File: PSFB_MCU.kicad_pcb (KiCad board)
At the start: 4 copper layers, 122.5 x 123.5 mm, 296 parts, among them Y1 16M

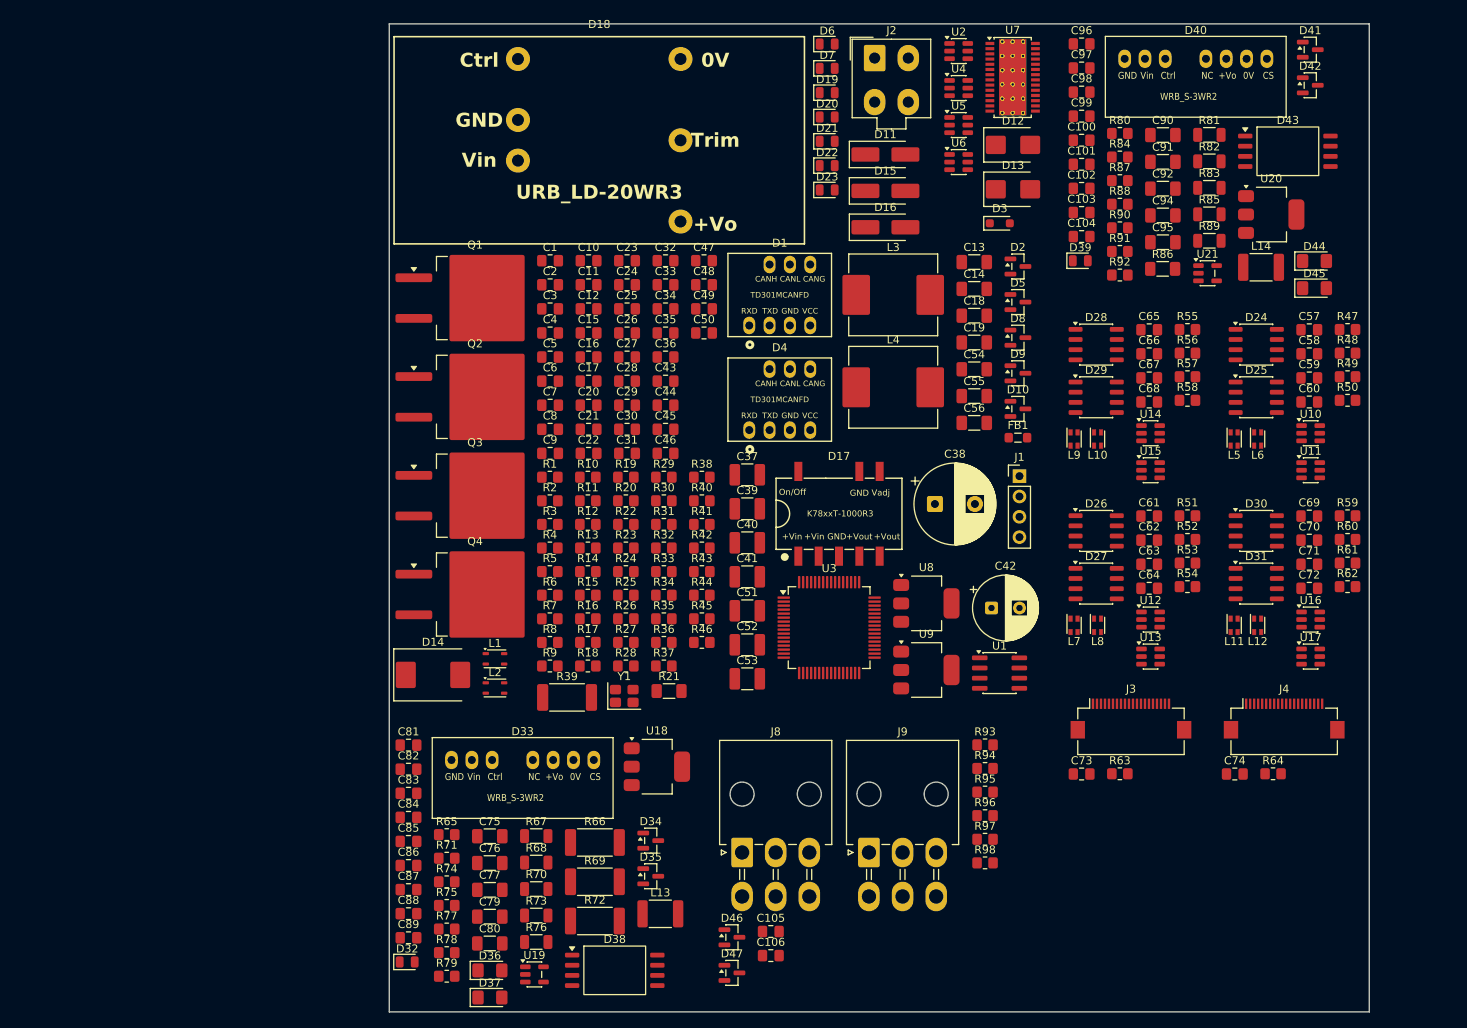
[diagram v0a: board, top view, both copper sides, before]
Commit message: VER1.0: раскидал компоненты на плате
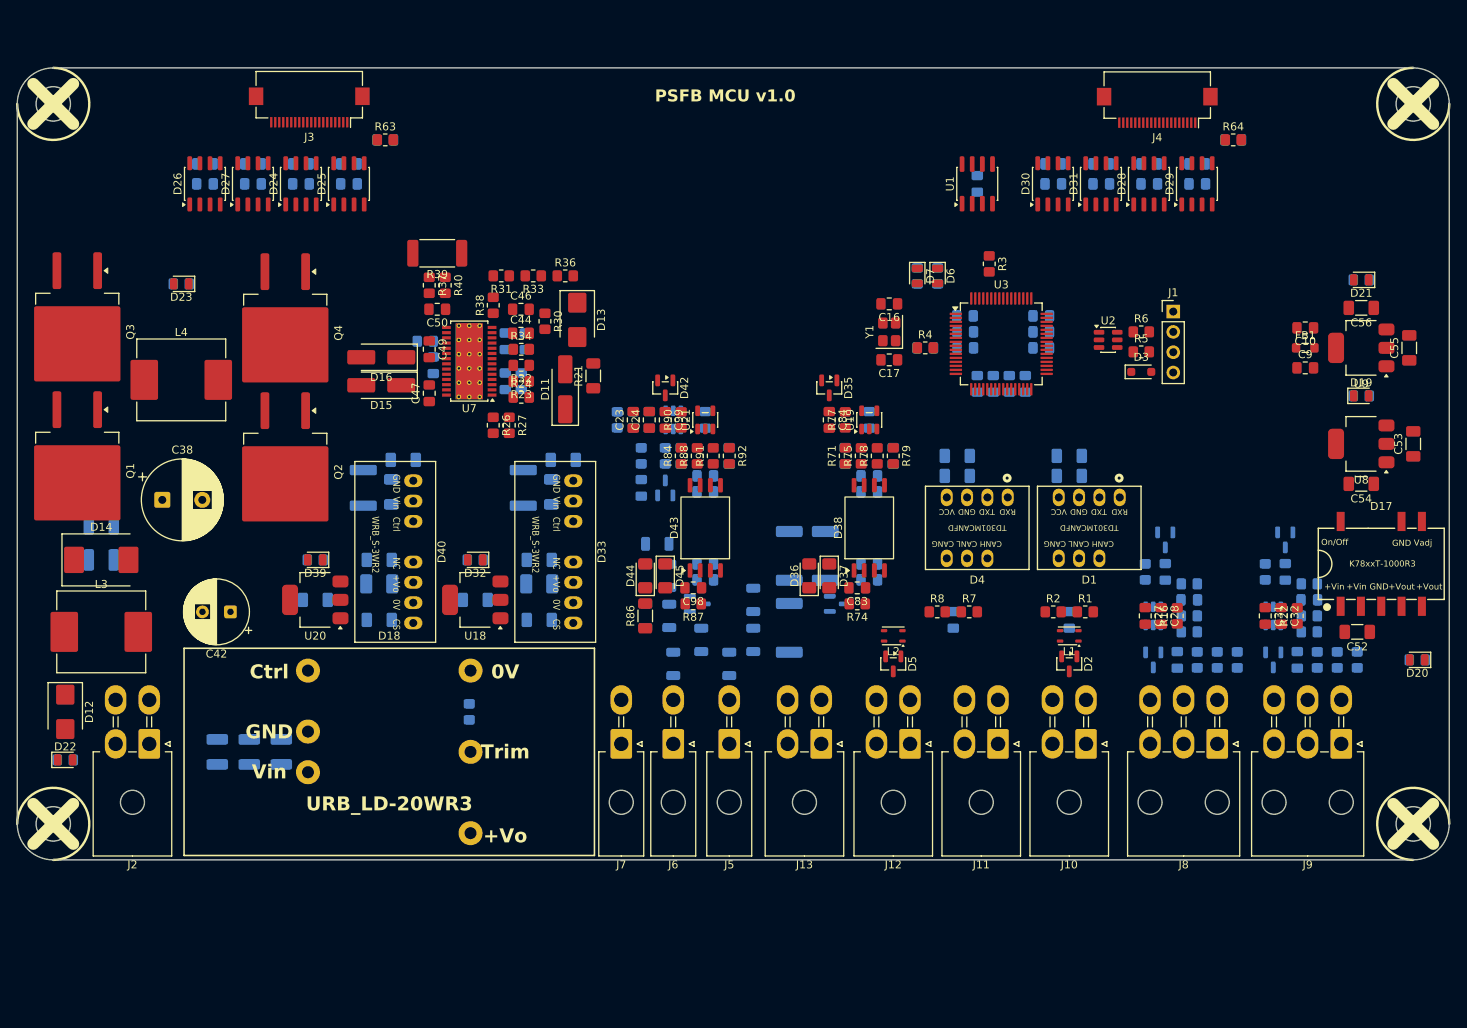
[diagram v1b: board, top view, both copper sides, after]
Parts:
- removed L10, L11, L12, L5, L6, L7, L8, L9: ~, Inductor_SMD:L_CommonModeChoke_Coilcraft_0805USB
- removed R47, R48, R49, R50, R51, R52, R53, R54, R55, R56, R57, R58, R59, R60, R61, R62: 0, Resistor_SMD:R_0805_2012Metric_Pad1.20x1.40mm_HandSolder
- removed U10, U11, U12, U13, U14, U15, U16, U17: ~, Package_TO_SOT_SMD:SOT-23-6
- added C78: 100u, Capacitor_Tantalum_SMD:CP_EIA-3528-21_Kemet-B_HandSolder, B.Cu at (101.2, 106.5)
- added C93: 100u, Capacitor_Tantalum_SMD:CP_EIA-3528-21_Kemet-B_HandSolder, B.Cu at (81.2, 106.5)
- added H1: MountingHole, MountingHole:MountingHole_4.3mm_M4, F.Cu at (40.5, 46.5)
- added H2: MountingHole, MountingHole:MountingHole_4.3mm_M4, F.Cu at (40.5, 136.5)
- added H3: MountingHole, MountingHole:MountingHole_4.3mm_M4, F.Cu at (210.5, 46.5)
- added H4: MountingHole, MountingHole:MountingHole_4.3mm_M4, F.Cu at (210.5, 136.5)
- added J10: ~, Connector_Molex:Molex_Mini-Fit_Jr_5569-04A2_2x02_P4.20mm_Horizontal, F.Cu at (169.6, 126.5)
- added J11: ~, Connector_Molex:Molex_Mini-Fit_Jr_5569-04A2_2x02_P4.20mm_Horizontal, F.Cu at (158.6, 126.5)
- added J12: ~, Connector_Molex:Molex_Mini-Fit_Jr_5569-04A2_2x02_P4.20mm_Horizontal, F.Cu at (147.6, 126.5)
- added J13: ~, Connector_Molex:Molex_Mini-Fit_Jr_5569-04A2_2x02_P4.20mm_Horizontal, F.Cu at (136.5, 126.5)
- added J5: ~, Connector_Molex:Molex_Mini-Fit_Jr_5569-02A2_2x01_P4.20mm_Horizontal, F.Cu at (125.0, 126.5)
- added J6: ~, Connector_Molex:Molex_Mini-Fit_Jr_5569-02A2_2x01_P4.20mm_Horizontal, F.Cu at (118.0, 126.5)
- added J7: ~, Connector_Molex:Molex_Mini-Fit_Jr_5569-02A2_2x01_P4.20mm_Horizontal, F.Cu at (111.5, 126.5)
- C1, C100, C101, C102, C103, C104, C105, C106, C11, C12, C13, C14, C15, C18, C19, C2, C20, C21, C22, C25, C26, C29, C3, C30, C33, C34, C35, C36, C37, C39, C4, C40, C41, C43, C45, C48, C5, C51, C57, C58, C59, C6, C60, C61, C62, C63, C64, C65, C66, C67, C68, C69, C7, C70, C71, C72, C73, C74, C75, C76, C77, C79, C8, C80, C81, C82, C85, C86, C87, C88, C89, C90, C91, C92, C94, C95, C96, C97, D10, D34, D41, D46, D47, D8, D9, L13, L14, R10, R11, R12, R13, R14, R15, R17, R18, R19, R20, R25, R28, R29, R35, R41, R42, R43, R44, R45, R46, R65, R66, R67, R68, R69, R70, R72, R73, R76, R80, R81, R82, R83, R85, R89, R9, R93, R94, R95, R96, R97, R98, U4, U5, U6: moved to B.Cu
- C38: value 100u -> 68u
- C52, C53: footprint Capacitor_SMD:C_1210_3225Metric_Pad1.33x2.70mm_HandSolder -> Capacitor_SMD:C_1206_3216Metric_Pad1.33x1.80mm_HandSolder
- J2: footprint Connector_Molex:Molex_Mini-Fit_Jr_5566-04A_2x02_P4.20mm_Vertical -> Connector_Molex:Molex_Mini-Fit_Jr_5569-04A2_2x02_P4.20mm_Horizontal
- moved D12 138.1 mm to (42.0, 122.5), turned to -90 degrees
- moved U20 128.8 mm to (73.2, 108.5), turned to 180 degrees
- moved J3 128.0 mm to (72.5, 47.0), turned to 180 degrees
- moved C58 127.8 mm to (71.5, 56.5)
- moved C57 127.7 mm to (71.5, 54.0)
- moved C62 126.2 mm to (59.5, 56.5)
- moved C61 126.0 mm to (59.5, 54.0)
- moved J2 124.8 mm to (52.5, 126.5), turned to 180 degrees
- moved C60 123.1 mm to (77.5, 56.5)
- moved C59 123.0 mm to (77.5, 54.0)
- moved C64 122.9 mm to (65.5, 56.5)
- moved C63 122.7 mm to (65.5, 54.0)
- moved R63 121.3 mm to (82.0, 51.0)
- moved D24 121.1 mm to (71.5, 56.5), turned to 90 degrees
- moved D22 120.8 mm to (42.0, 128.5)
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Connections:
- C101 pad 2: +3.3VP -> +3V3
- C102 pad 1: +3.3VP -> +3V3
- C95 pad 2: +3.3VP -> +3V3
- D24 pad 6: Net-(D24-A) -> /Connector_channel_1/PWM_L1_P
- D24 pad 7: Net-(D24-B) -> /Connector_channel_1/PWM_L1_N
- D25 pad 6: Net-(D25-A) -> /Connector_channel_1/PWM_H1_P
- D25 pad 7: Net-(D25-B) -> /Connector_channel_1/PWM_H1_N
- D26 pad 6: Net-(D26-A) -> /Connector_channel_1/PWM_L2_P
- D26 pad 7: Net-(D26-B) -> /Connector_channel_1/PWM_L2_N
- D27 pad 6: Net-(D27-A) -> /Connector_channel_1/PWM_H2_P
- D27 pad 7: Net-(D27-B) -> /Connector_channel_1/PWM_H2_N
- D28 pad 6: Net-(D28-A) -> /Connector_channel_2/PWM_L1_P
- D28 pad 7: Net-(D28-B) -> /Connector_channel_2/PWM_L1_N
- D29 pad 6: Net-(D29-A) -> /Connector_channel_2/PWM_H1_P
- D29 pad 7: Net-(D29-B) -> /Connector_channel_2/PWM_H1_N
- D30 pad 6: Net-(D30-A) -> /Connector_channel_2/PWM_L2_P
- D30 pad 7: Net-(D30-B) -> /Connector_channel_2/PWM_L2_N
- D31 pad 6: Net-(D31-A) -> /Connector_channel_2/PWM_H2_P
- D31 pad 7: Net-(D31-B) -> /Connector_channel_2/PWM_H2_N
- D39 pad 2: +3.3VP -> +3V3
- D41 pad 2: +3.3VP -> +3V3
- D43 pad 1: +3.3VP -> +3V3
- J2 pad 1: VIN -> GND_IN
- J2 pad 4: GND_IN -> VIN
- U20 pad 2: +3.3VP -> +3V3
- U3 pad 61: unconnected-(U3-PB8-Pad61) -> /OverVoltage
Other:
- board size 122.5 x 123.5 mm -> 179 x 99 mm
- board text added: "PSFB MCU v1.0"
